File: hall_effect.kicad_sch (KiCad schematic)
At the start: 11 parts, among them U2 OPA196xDGK, U3 SM351LT, U4 OPA196xDGK

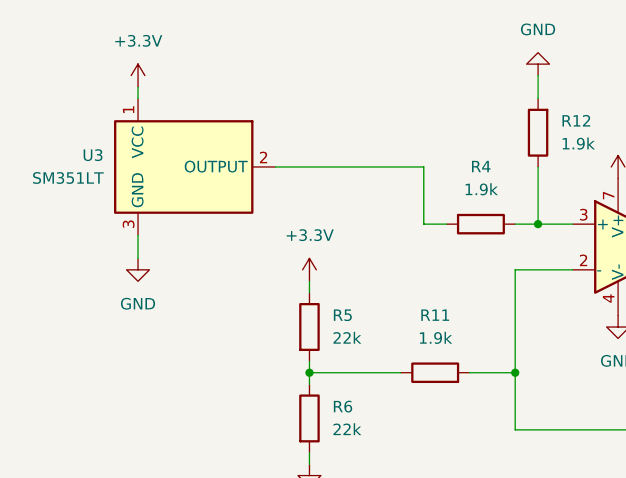
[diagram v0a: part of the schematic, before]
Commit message: layout work
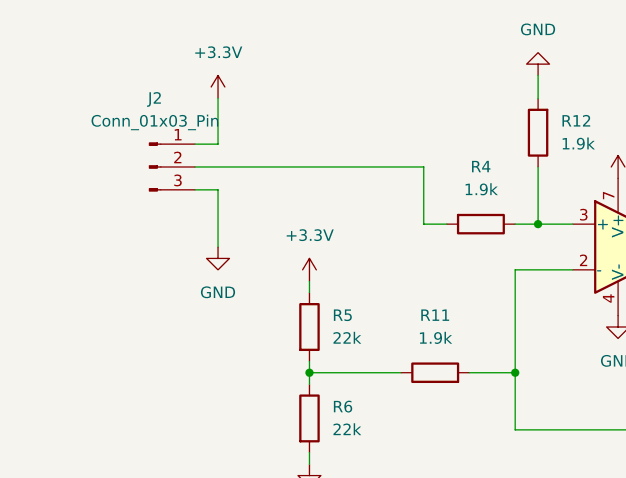
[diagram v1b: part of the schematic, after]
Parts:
- removed U3: SM351LT, Package_TO_SOT_SMD:SOT-23, symbol Sensor_Magnetic:SM351LT
- added J2: Conn_01x03_Pin, Connector_PinHeader_2.54mm:PinHeader_1x03_P2.54mm_Vertical, symbol Connector:Conn_01x03_Pin
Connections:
- net +3.3V: now also J2.1 (Pin_1)
- net GND: now also J2.3 (Pin_3)
- net at R4.2: now also J2.2 (Pin_2)
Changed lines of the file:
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@@
 	(wire
 		(pts
-			(xy 73.66 59.69) (xy 90.17 59.69)
+			(xy 67.31 52.07) (xy 67.31 57.15)
 		)
 		(stroke
@@
 	(wire
 		(pts
+			(xy 67.31 57.15) (xy 64.77 57.15)
+		)
+		(stroke
+			(width 0)
+			(type default)
+		)
+	)
+	(wire
+		(pts
 			(xy 138.43 93.98) (xy 138.43 96.52)
 		)
@@
 	(wire
 		(pts
-			(xy 58.42 50.8) (xy 58.42 52.07)
+			(xy 64.77 59.69) (xy 90.17 59.69)
 		)
 		(stroke
@@
 	(wire
 		(pts
-			(xy 58.42 67.31) (xy 58.42 69.85)
-		)
-		(stroke
-			(width 0)
-			(type default)
-		)
-	)
-	(wire
-		(pts
 			(xy 102.87 49.53) (xy 102.87 52.07)
 		)
@@
 	(wire
 		(pts
+			(xy 67.31 62.23) (xy 64.77 62.23)
+		)
+		(stroke
+			(width 0)
+			(type default)
+		)
+	)
+	(wire
+		(pts
 			(xy 100.33 66.04) (xy 102.87 66.04)
 		)
@@
 		(pts
 			(xy 100.33 88.9) (xy 113.03 88.9)
+		)
+		(stroke
+			(width 0)
+			(type default)
+		)
+	)
+	(wire
+		(pts
+			(xy 67.31 68.58) (xy 67.31 62.23)
 		)
 		(stroke
@@
 	(symbol
 		(lib_id "power:GND")
-		(at 58.42 69.85 0)
+		(at 67.31 68.58 0)
 		(unit 1)
 		(exclude_from_sim no)
@@
 		(fields_autoplaced yes)
 		(property "Reference" "#PWR027"
-			(at 58.42 76.2 0)
+			(at 67.31 74.93 0)
 			(effects
 				(font
@@
 		)
 		(property "Value" "GND"
-			(at 58.42 74.93 0)
+			(at 67.31 73.66 0)
 			(effects
 				(font
@@
 		)
 		(property "Footprint" ""
-			(at 58.42 69.85 0)
+			(at 67.31 68.58 0)
 			(effects
 				(font
@@
 		)
 		(property "Datasheet" ""
-			(at 58.42 69.85 0)
+			(at 67.31 68.58 0)
 			(effects
 				(font
@@
 		)
 		(property "Description" "Power symbol creates a global label with name \"GND\" , ground"
-			(at 58.42 69.85 0)
+			(at 67.31 68.58 0)
 			(effects
 				(font
@@
 	)
 	(symbol
+		(lib_id "Connector:Conn_01x03_Pin")
+		(at 59.69 59.69 0)
+		(unit 1)
+		(exclude_from_sim no)
+		(in_bom yes)
+		(on_board yes)
+		(dnp no)
+		(fields_autoplaced yes)
+		(property "Reference" "J2"
+			(at 60.325 52.07 0)
+			(effects
+				(font
+					(size 1.27 1.27)
+				)
+			)
+		)
+		(property "Value" "Conn_01x03_Pin"
+			(at 60.325 54.61 0)
+			(effects
+				(font
+					(size 1.27 1.27)
+				)
+			)
+		)
+		(property "Footprint" "Connector_PinHeader_2.54mm:PinHeader_1x03_P2.54mm_Vertical"
+			(at 59.69 59.69 0)
+			(effects
+				(font
+					(size 1.27 1.27)
+				)
+				(hide yes)
+			)
+		)
+		(property "Datasheet" "~"
+			(at 59.69 59.69 0)
+			(effects
+				(font
+					(size 1.27 1.27)
+				)
+				(hide yes)
+			)
+		)
+		(property "Description" "Generic connector, single row, 01x03, script generated"
+			(at 59.69 59.69 0)
+			(effects
+				(font
+					(size 1.27 1.27)
+				)
+				(hide yes)
+			)
+		)
+		(pin "3"
+		)
+		(pin "1"
+		)
+		(pin "2"
+		)
+		(instances
+			(project ""
+				(path "/35c074f0-8545-4dc1-a57d-3ef0bc7d9188/ce5cb751-dcc9-43da-9e85-60783f09935d"
+					(reference "J2")
+					(unit 1)
+				)
+			)
+		)
+	)
+	(symbol
 		(lib_id "Device:R")
 		(at 102.87 55.88 180)
@@
 	)
 	(symbol
-		(lib_id "Sensor_Magnetic:SM351LT")
-		(at 63.5 59.69 0)
-		(unit 1)
-		(exclude_from_sim no)
-		(in_bom yes)
-		(on_board yes)
-		(dnp no)
-		(fields_autoplaced yes)
-		(property "Reference" "U3"
-			(at 54.61 58.4199 0)
-			(effects
-				(font
-					(size 1.27 1.27)
-				)
-				(justify right)
-			)
-		)
-		(property "Value" "SM351LT"
-			(at 54.61 60.9599 0)
-			(effects
-				(font
-					(size 1.27 1.27)
-				)
-				(justify right)
-			)
-		)
-		(property "Footprint" "Package_TO_SOT_SMD:SOT-23"
-			(at 62.23 59.69 0)
-			(effects
-				(font
-					(size 1.27 1.27)
-				)
-				(hide yes)
-			)
-		)
-		(property "Datasheet" "https://sensing.honeywell.com/honeywell-sensing-nanopower-series-product-sheet-50095501-a-en.pdf"
-			(at 62.23 59.69 0)
-			(effects
-				(font
-					(size 1.27 1.27)
-				)
-				(hide yes)
-			)
-		)
-		(property "Description" "Hall Effect Switch, SOT-23"
-			(at 63.5 59.69 0)
-			(effects
-				(font
-					(size 1.27 1.27)
-				)
-				(hide yes)
-			)
-		)
-		(pin "2"
-		)
-		(pin "1"
-		)
-		(pin "3"
-		)
-		(instances
-			(project ""
-				(path "/35c074f0-8545-4dc1-a57d-3ef0bc7d9188/ce5cb751-dcc9-43da-9e85-60783f09935d"
-					(reference "U3")
-					(unit 1)
-				)
-			)
-		)
-	)
-	(symbol
 		(lib_id "Amplifier_Operational:OPA196xDGK")
 		(at 151.13 71.12 0)
@@
 	(symbol
 		(lib_id "power:+3.3V")
-		(at 58.42 50.8 0)
+		(at 67.31 52.07 0)
 		(unit 1)
 		(exclude_from_sim no)
@@
 		(fields_autoplaced yes)
 		(property "Reference" "#PWR026"
-			(at 58.42 54.61 0)
+			(at 67.31 55.88 0)
 			(effects
 				(font
@@
 		)
 		(property "Value" "+3.3V"
-			(at 58.42 45.72 0)
+			(at 67.31 46.99 0)
 			(effects
 				(font
@@
 		)
 		(property "Footprint" ""
-			(at 58.42 50.8 0)
+			(at 67.31 52.07 0)
 			(effects
 				(font
@@
 		)
 		(property "Datasheet" ""
-			(at 58.42 50.8 0)
+			(at 67.31 52.07 0)
 			(effects
 				(font
@@
 		)
 		(property "Description" "Power symbol creates a global label with name \"+3.3V\""
-			(at 58.42 50.8 0)
-			(effects
-				(font
+			(at 67.31 52.07 0)
+			(effects
+				(font
